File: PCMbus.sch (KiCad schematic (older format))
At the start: 10 parts

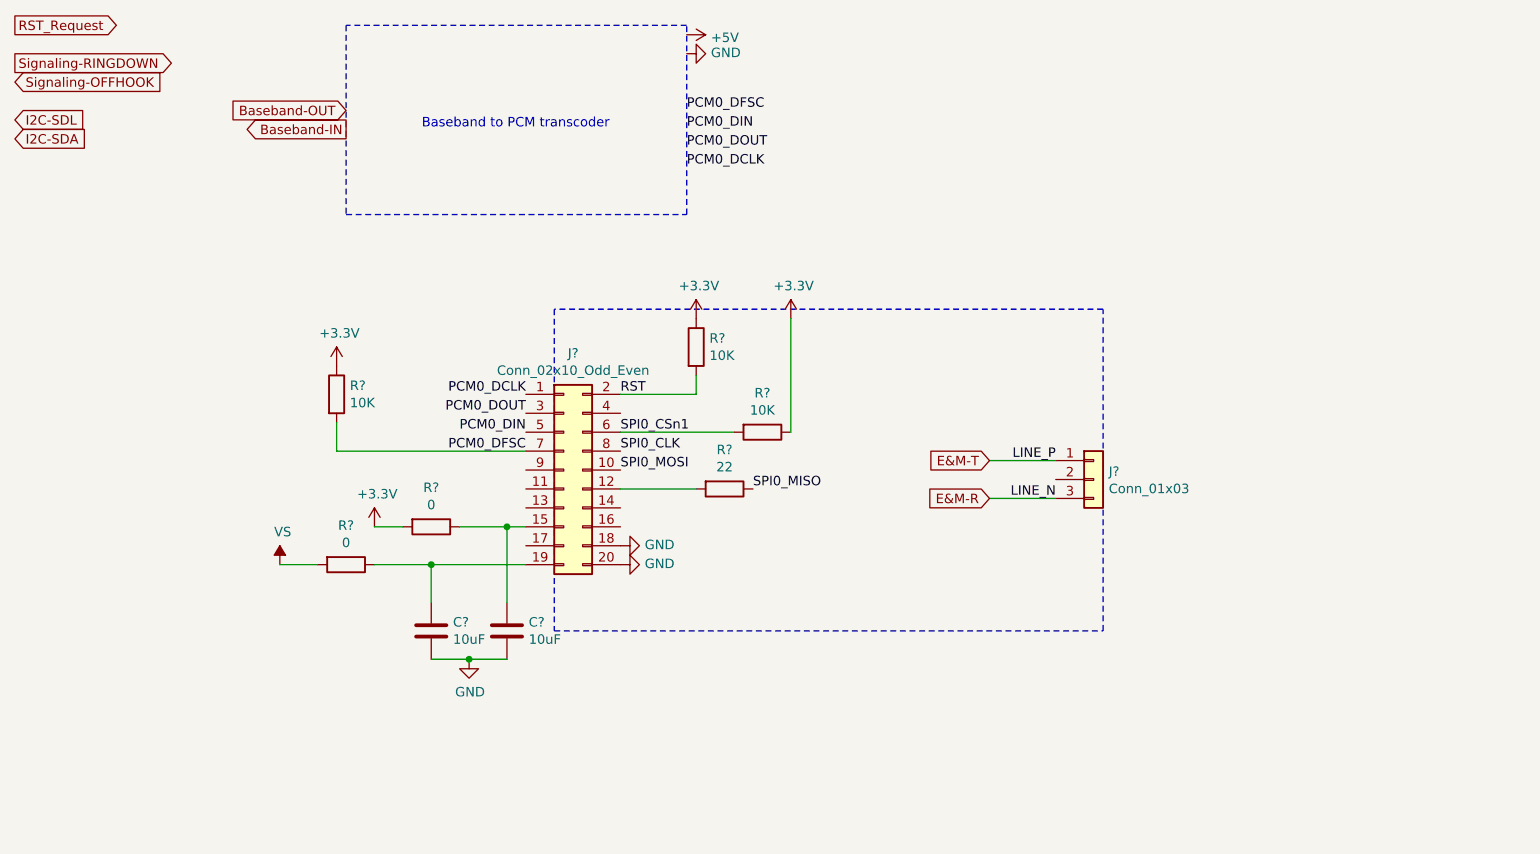
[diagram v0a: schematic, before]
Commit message: updates
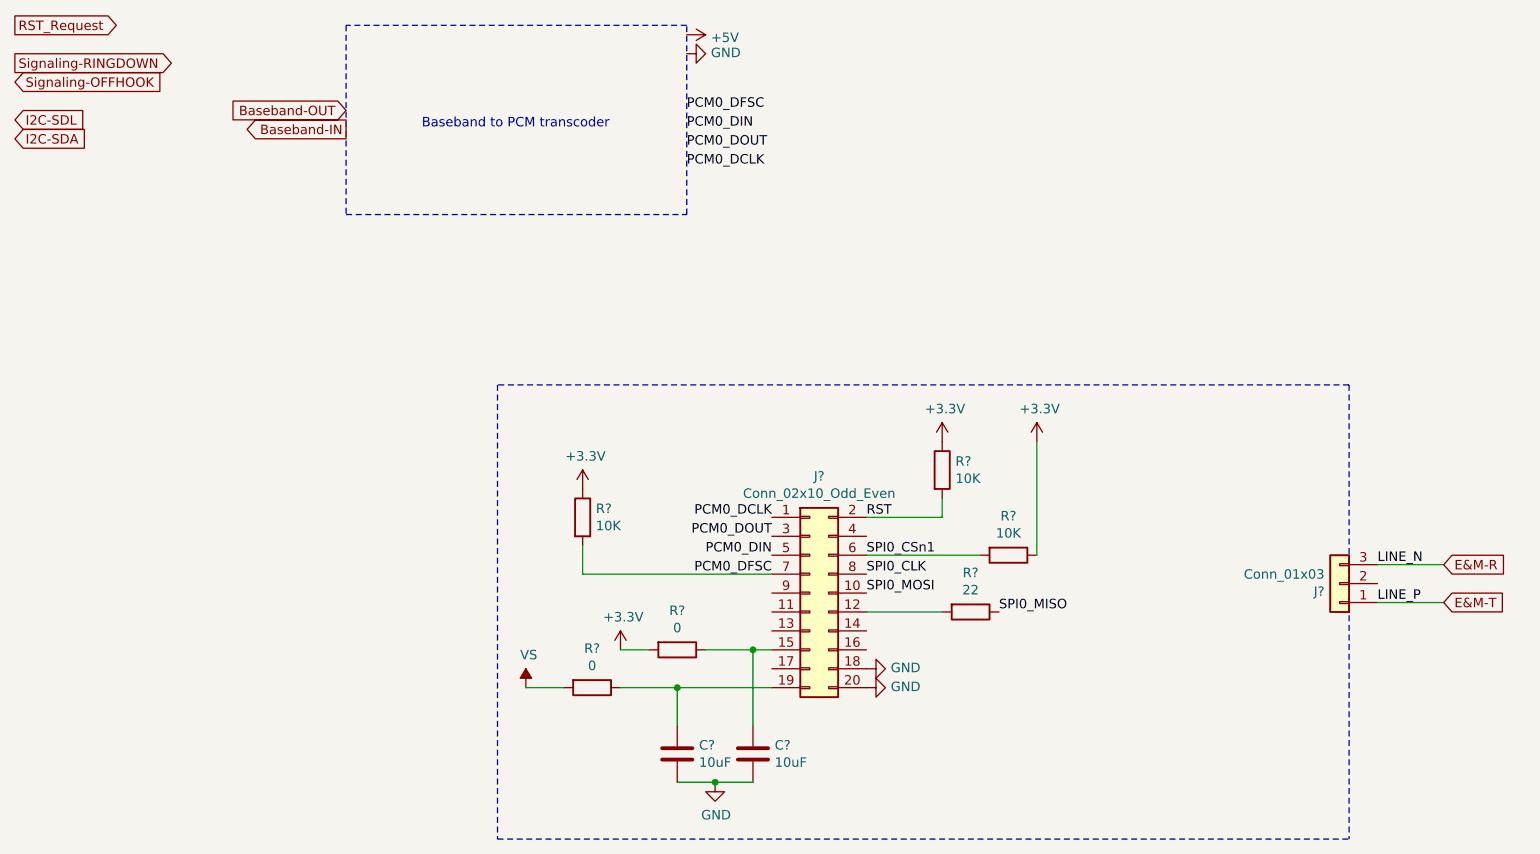
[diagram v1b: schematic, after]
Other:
- moved on the sheet: C?, J?, R?
